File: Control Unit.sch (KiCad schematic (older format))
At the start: 0 parts

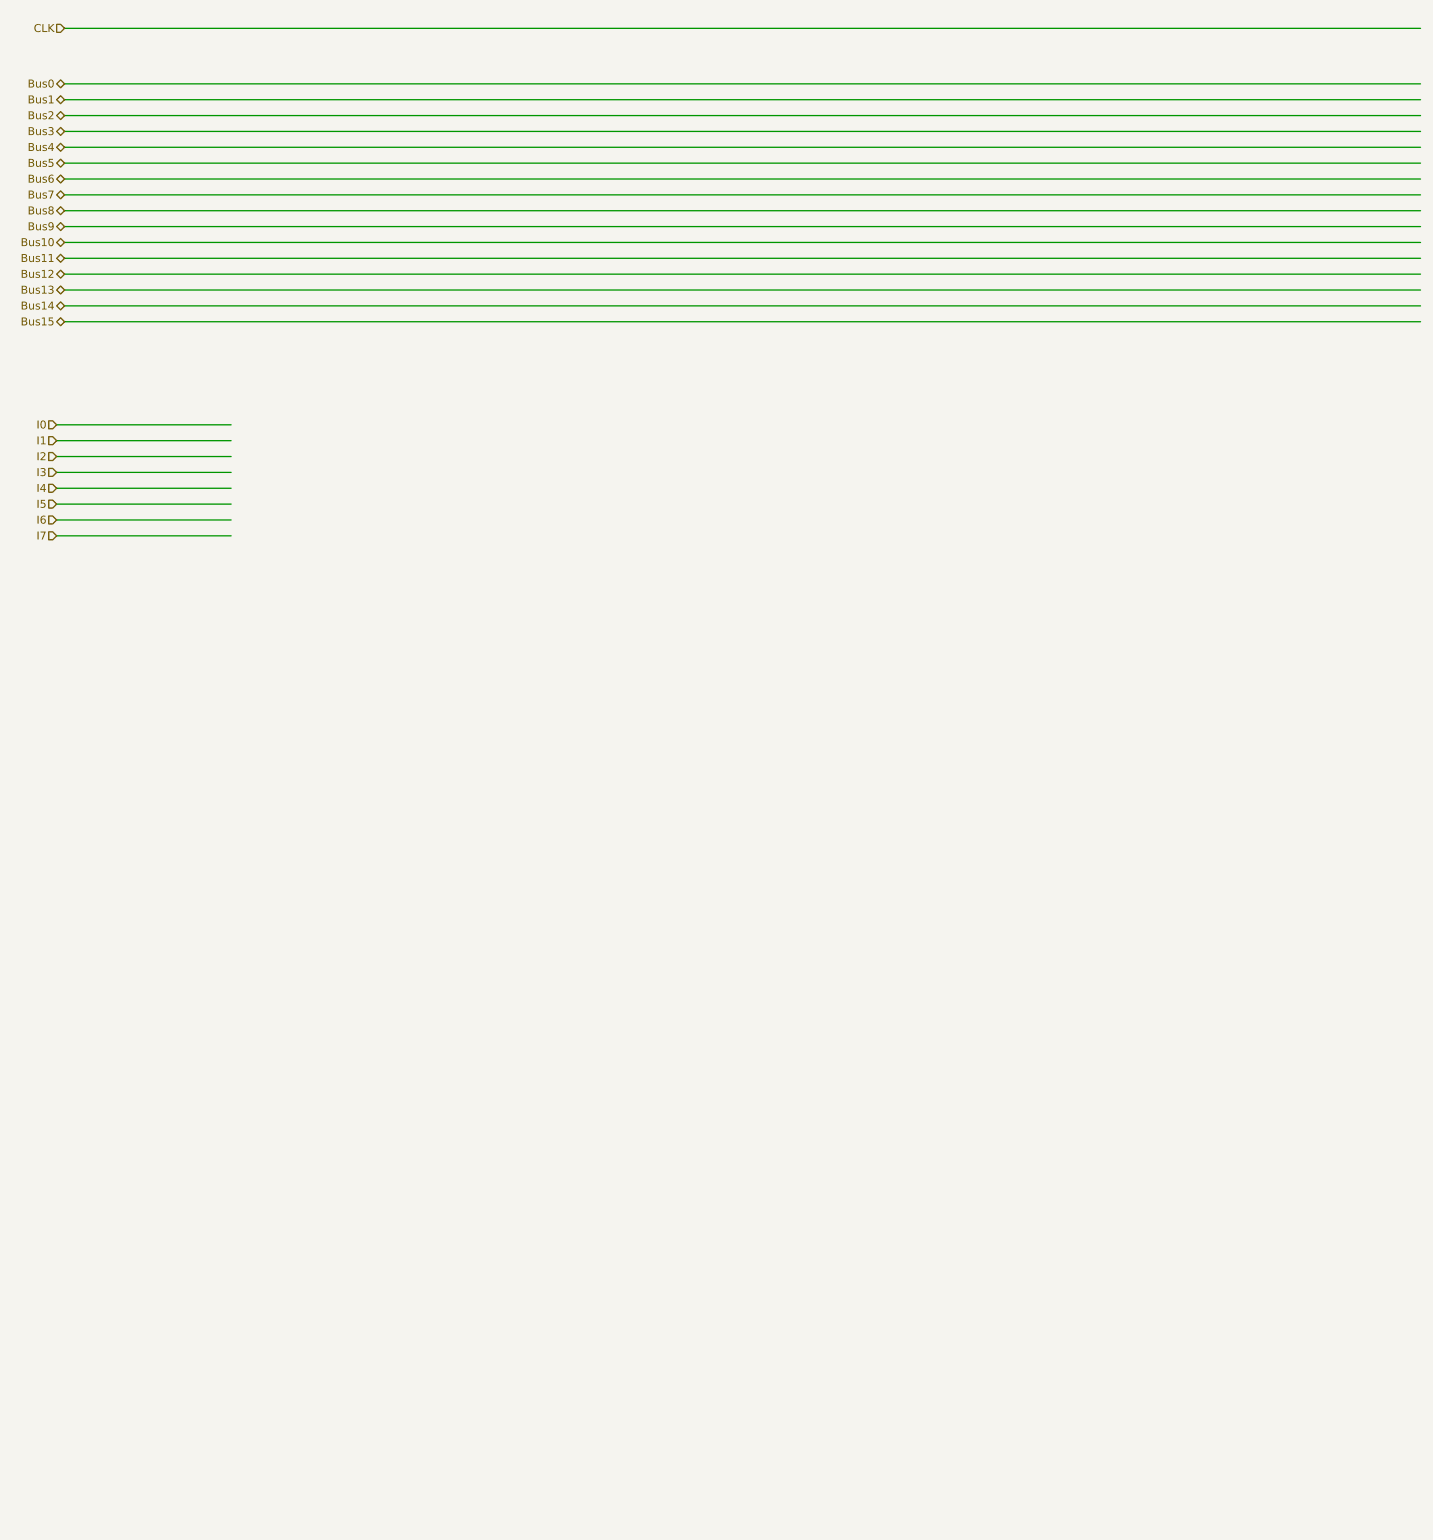
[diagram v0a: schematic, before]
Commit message: made the CU , need to change the IR
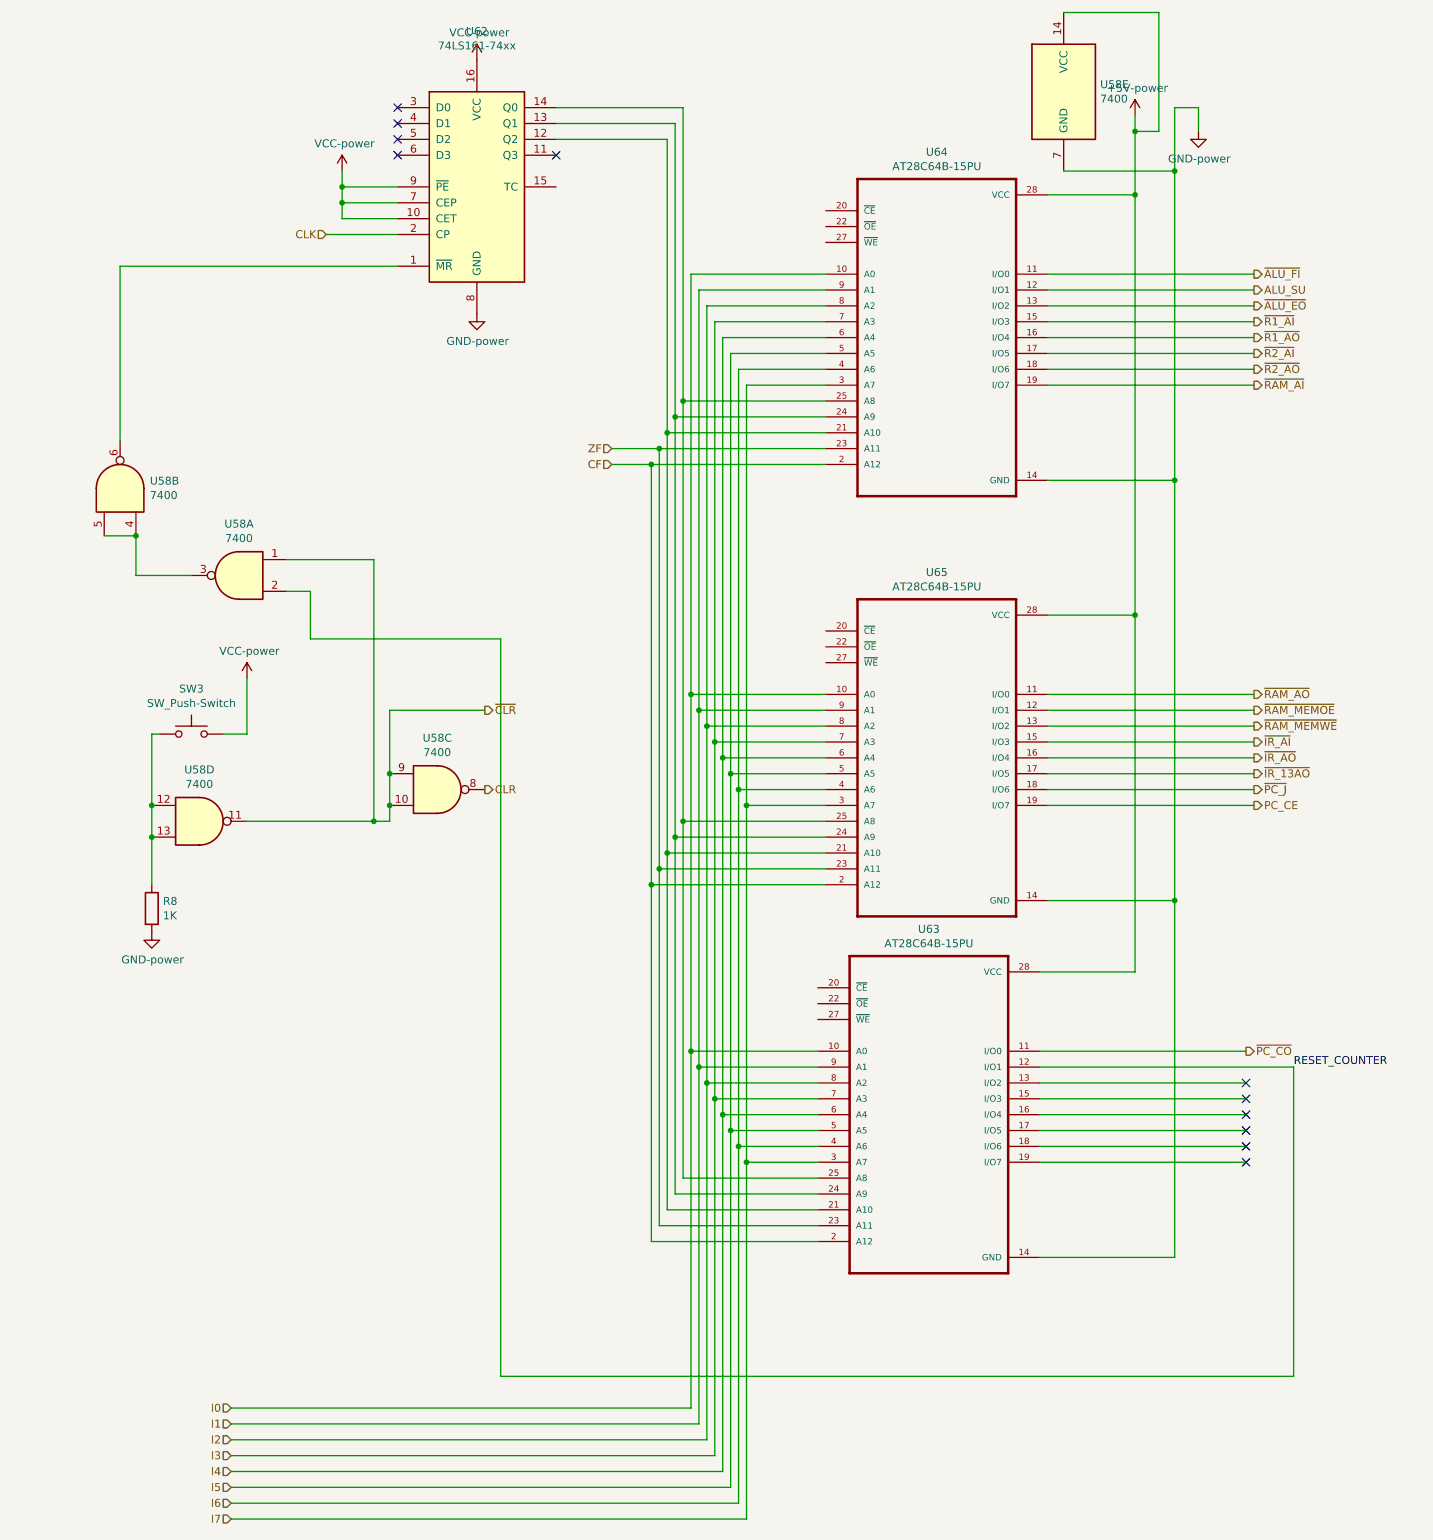
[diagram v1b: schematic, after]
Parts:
- added R8: 1K, Resistor_THT:R_Axial_DIN0204_L3.6mm_D1.6mm_P7.62mm_Horizontal, symbol 16bitCpu-rescue:R-Device
- added SW3: SW_Push-Switch, Button_Switch_THT:SW_PUSH-12mm, symbol 16bitCpu-rescue:SW_Push-Switch
- added U58: 7400, Package_DIP:DIP-14_W7.62mm, symbol 74xx:7400
- added U62: 74LS161-74xx, Package_DIP:DIP-16_W7.62mm, symbol 16bitCpu-rescue:74LS161-74xx
- added U63, U64, U65: AT28C64B-15PU, ROM:ZIF-AT28C64B-15PU, symbol AT28C64B-15PU:AT28C64B-15PU
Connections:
- net labels added: +5V-power, ALU_SU, CF, CLR, GND-power, PC_CE, RESET_COUNTER, VCC-power, ZF, ~ALU_EO, ~ALU_FI, ~CLR, ~IR_13AO, ~IR_AI, ~IR_AO, ~PC_CO, ~PC_J, ~R1_AI, ~R1_AO, ~R2_AI, ~R2_AO, ~RAM_AI, ~RAM_AO, ~RAM_MEMOE, ~RAM_MEMWE
- net labels removed: Bus0, Bus1, Bus10, Bus11, Bus12, Bus13, Bus14, Bus15, Bus2, Bus3, Bus4, Bus5, Bus6, Bus7, Bus8, Bus9
- wire segments 25 -> 165
- no-connect marks 0 -> 11
